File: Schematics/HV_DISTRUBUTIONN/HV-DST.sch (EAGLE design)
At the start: 37 parts

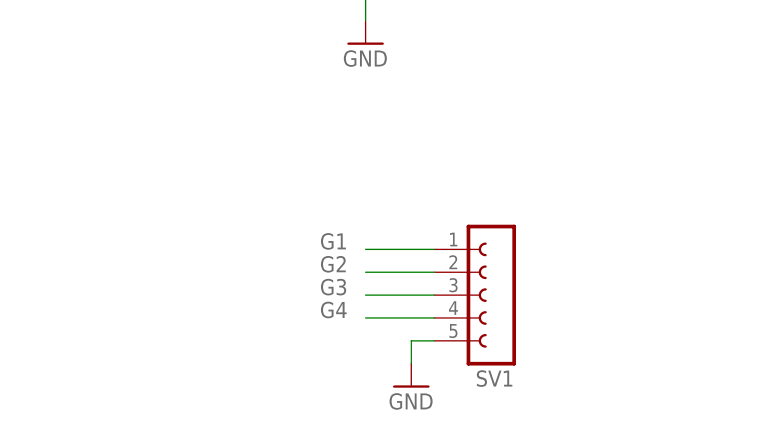
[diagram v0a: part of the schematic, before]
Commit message: Finished routing
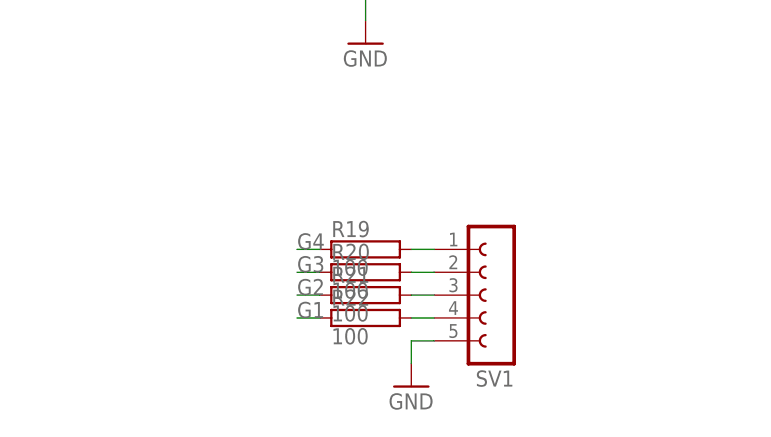
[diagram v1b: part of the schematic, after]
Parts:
- added R19, R20, R21, R22: 100, resistor-power:RRS1/4
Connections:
- new net N$15: R20.2, SV1.2
- new net N$17: R21.2, SV1.3
- new net N$18: R22.2, SV1.4
- new net N$7: R19.2, SV1.1
- net G1: now also R22.1; no longer SV1.1
- net G2: now also R21.1; no longer SV1.2
- net G3: now also R20.1; no longer SV1.3
- net G4: now also R19.1; no longer SV1.4
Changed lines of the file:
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@@
 <part name="SV1" library="con-lsta" deviceset="FE05-1" device=""/>
 <part name="GND7" library="supply1" deviceset="GND" device=""/>
+<part name="R19" library="resistor-power" deviceset="R" device="RS1/4" value="100"/>
+<part name="R20" library="resistor-power" deviceset="R" device="RS1/4" value="100"/>
+<part name="R21" library="resistor-power" deviceset="R" device="RS1/4" value="100"/>
+<part name="R22" library="resistor-power" deviceset="R" device="RS1/4" value="100"/>
 </parts>
 <sheets>
@@
 <instance part="SV1" gate="G$1" x="81.28" y="30.48" rot="R180"/>
 <instance part="GND7" gate="1" x="71.12" y="20.32"/>
+<instance part="R19" gate="G$1" x="66.04" y="35.56"/>
+<instance part="R20" gate="G$1" x="66.04" y="33.02"/>
+<instance part="R21" gate="G$1" x="66.04" y="30.48"/>
+<instance part="R22" gate="G$1" x="66.04" y="27.94"/>
 </instances>
 <busses>
@@
 </segment>
 <segment>
-<pinref part="SV1" gate="G$1" pin="1"/>
-<wire x1="73.66" y1="35.56" x2="66.04" y2="35.56" width="0.1524" layer="91"/>
-<label x="60.96" y="35.56" size="1.778" layer="95"/>
+<pinref part="R22" gate="G$1" pin="1"/>
+<wire x1="60.96" y1="27.94" x2="58.42" y2="27.94" width="0.1524" layer="91"/>
+<label x="58.42" y="27.94" size="1.778" layer="95"/>
 </segment>
 </net>
@@
 </segment>
 <segment>
-<pinref part="SV1" gate="G$1" pin="2"/>
-<wire x1="73.66" y1="33.02" x2="66.04" y2="33.02" width="0.1524" layer="91"/>
-<label x="60.96" y="33.02" size="1.778" layer="95"/>
+<pinref part="R21" gate="G$1" pin="1"/>
+<wire x1="60.96" y1="30.48" x2="58.42" y2="30.48" width="0.1524" layer="91"/>
+<label x="58.42" y="30.48" size="1.778" layer="95"/>
 </segment>
 </net>
@@
 </segment>
 <segment>
-<pinref part="SV1" gate="G$1" pin="4"/>
-<wire x1="73.66" y1="27.94" x2="66.04" y2="27.94" width="0.1524" layer="91"/>
-<label x="60.96" y="27.94" size="1.778" layer="95"/>
+<pinref part="R19" gate="G$1" pin="1"/>
+<wire x1="60.96" y1="35.56" x2="58.42" y2="35.56" width="0.1524" layer="91"/>
+<label x="58.42" y="35.56" size="1.778" layer="95"/>
 </segment>
 </net>
@@
 </segment>
 <segment>
-<pinref part="SV1" gate="G$1" pin="3"/>
-<wire x1="73.66" y1="30.48" x2="66.04" y2="30.48" width="0.1524" layer="91"/>
-<label x="60.96" y="30.48" size="1.778" layer="95"/>
+<pinref part="R20" gate="G$1" pin="1"/>
+<wire x1="60.96" y1="33.02" x2="58.42" y2="33.02" width="0.1524" layer="91"/>
+<label x="58.42" y="33.02" size="1.778" layer="95"/>
 </segment>
 </net>
@@
 </segment>
 </net>
+<net name="N$7" class="0">
+<segment>
+<pinref part="SV1" gate="G$1" pin="1"/>
+<pinref part="R19" gate="G$1" pin="2"/>
+<wire x1="73.66" y1="35.56" x2="71.12" y2="35.56" width="0.1524" layer="91"/>
+</segment>
+</net>
+<net name="N$15" class="0">
+<segment>
+<pinref part="SV1" gate="G$1" pin="2"/>
+<pinref part="R20" gate="G$1" pin="2"/>
+<wire x1="73.66" y1="33.02" x2="71.12" y2="33.02" width="0.1524" layer="91"/>
+</segment>
+</net>
+<net name="N$17" class="0">
+<segment>
+<pinref part="SV1" gate="G$1" pin="3"/>
+<pinref part="R21" gate="G$1" pin="2"/>
+<wire x1="73.66" y1="30.48" x2="71.12" y2="30.48" width="0.1524" layer="91"/>
+</segment>
+</net>
+<net name="N$18" class="0">
+<segment>
+<pinref part="SV1" gate="G$1" pin="4"/>
+<pinref part="R22" gate="G$1" pin="2"/>
+<wire x1="73.66" y1="27.94" x2="71.12" y2="27.94" width="0.1524" layer="91"/>
+</segment>
+</net>
